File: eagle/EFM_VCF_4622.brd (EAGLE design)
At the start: 101.6 x 80.8 mm, 61 parts, among them IC1 LM13700N, Q1 2N3906, Q10 2N3904, Q11 2N3904, Q12 2N3904, Q13 2N3904, Q2 2N3904, Q3 2N3904, Q4 2N3904, Q5 2N3904, Q6 2N3904, Q7 2N3904, Q8 2N3904, Q9 2N3904

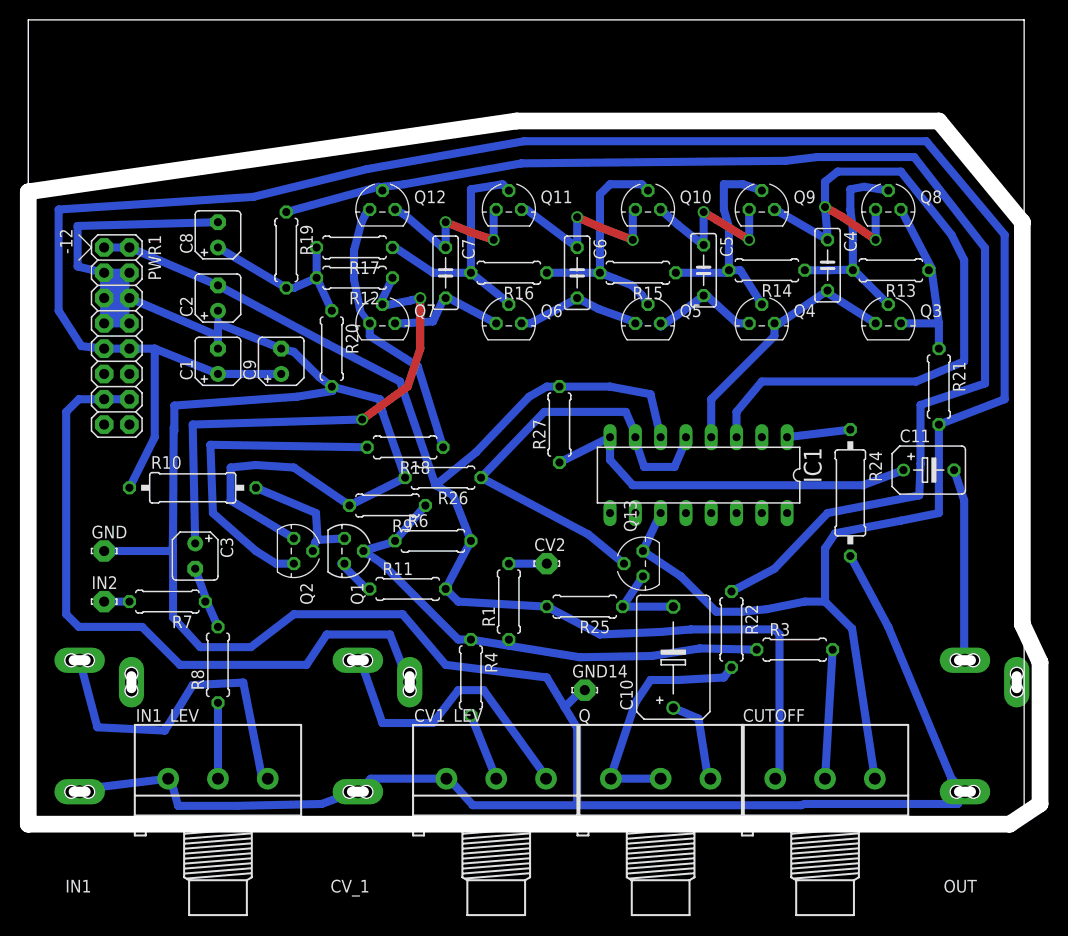
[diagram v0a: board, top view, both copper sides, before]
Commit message: tidied still more
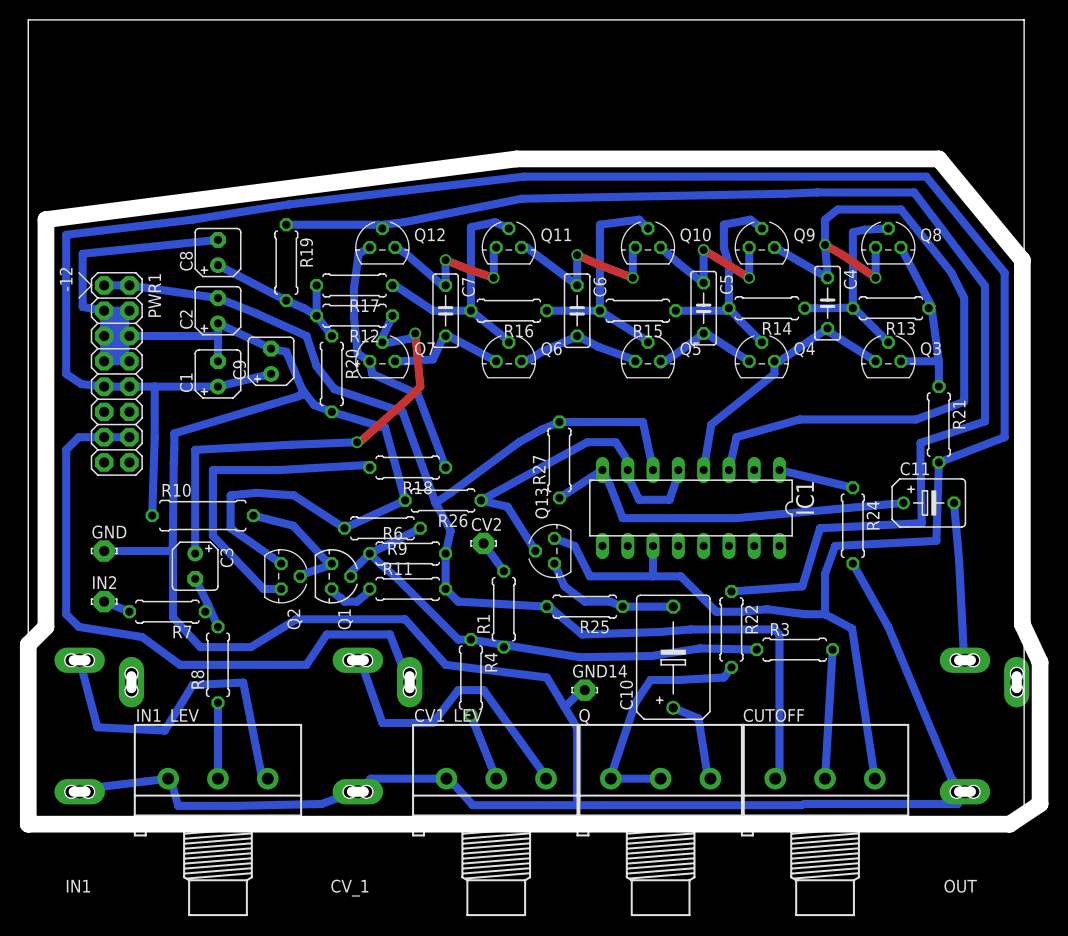
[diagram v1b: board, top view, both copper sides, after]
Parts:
- R10: device rcl:0309/12 -> rcl:0309/10
- R24: device rcl:0309/12 -> rcl:0207/7
- moved Q13 8.98 mm to (52.8, 26.7)
- moved CV2 6.67 mm to (45.7, 27.4)
- moved C4 3.81 mm to (80.3, 51.6)
- moved C6 3.81 mm to (55.1, 50.8)
- moved C7 3.81 mm to (41.9, 50.8)
- moved Q10 3.81 mm to (62.2, 57.1)
- moved Q11 3.81 mm to (48.3, 57.1)
- moved Q12 3.81 mm to (35.6, 57.1)
- moved Q3 3.81 mm to (86.4, 45.7)
- moved Q4 3.81 mm to (73.7, 45.7)
- moved Q5 3.81 mm to (62.2, 45.7)
- moved Q6 3.81 mm to (48.3, 45.7)
- moved Q7 3.81 mm to (35.6, 45.7)
- moved Q8 3.81 mm to (86.4, 57.1)
- moved Q9 3.81 mm to (73.7, 57.1)
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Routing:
- net N$19: track 46.3 -> 36.0 mm
- net GND: track 328.1 -> 321.0 mm
- net N$35: track 8.74 -> 14.0 mm
- net N$55: track 71.2 -> 66.8 mm
- net -12V: track 137.0 -> 132.7 mm
- net +12V: track 243.7 -> 247.9 mm
- net N$7: track 51.0 -> 47.5 mm
- net N$31: track 19.5 -> 16.0 mm
- net N$27: track 4.23 -> 5.46 mm
- net N$25: track 17.9 -> 16.7 mm
- net N$1: track 6.40 -> 7.58 mm
- net N$3: track 32.5 -> 31.6 mm
- net N$44: track 21.9 -> 21.1 mm
- net N$4: track 27.7 -> 27.1 mm
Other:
- outline, holes or cut-outs redrawn
